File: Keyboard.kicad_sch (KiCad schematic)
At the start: 180 parts, among them SW1 SW_Push, SW10 SW_Push, SW11 SW_Push, SW12 SW_Push, SW13 SW_Push, SW14 SW_Push, SW15 SW_Push, SW16 SW_Push, SW17 SW_Push, SW18 SW_Push, SW19 SW_Push, SW2 SW_Push, SW20 SW_Push, SW21 SW_Push, SW22 SW_Push, SW23 SW_Push, SW24 SW_Push, SW25 SW_Push, SW26 SW_Push, SW27 SW_Push, SW28 SW_Push, SW29 SW_Push, SW3 SW_Push, SW30 SW_Push, SW31 SW_Push, SW32 SW_Push, SW33 SW_Push, SW34 SW_Push, SW35 SW_Push, SW36 SW_Push, SW37 SW_Push, SW38 SW_Push, SW39 SW_Push, SW4 SW_Push, SW40 SW_Push, SW41 SW_Push, SW42 SW_Push, SW43 SW_Push, SW44 SW_Push, SW45 SW_Push, SW46 SW_Push, SW47 SW_Push, SW48 SW_Push, SW49 SW_Push, SW5 SW_Push, SW50 SW_Push, SW51 SW_Push, SW52 SW_Push, SW53 SW_Push, SW54 SW_Push, SW55 SW_Push, SW56 SW_Push, SW57 SW_Push, SW58 SW_Push, SW59 SW_Push, SW6 SW_Push, SW60 SW_Push, SW61 SW_Push, SW62 SW_Push, SW63 SW_Push, SW64 SW_Push, SW65 SW_Push, SW66 SW_Push, SW67 SW_Push, SW68 SW_Push, SW69 SW_Push, SW7 SW_Push, SW70 SW_Push, SW71 SW_Push, SW72 SW_Push, SW73 SW_Push, SW74 SW_Push, SW75 SW_Push, SW76 SW_Push, SW77 SW_Push, SW78 SW_Push, SW79 SW_Push, SW8 SW_Push, SW80 SW_Push, SW81 SW_Push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

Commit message: updated footprints, didnt rlly seem to work lol
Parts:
- SW1, SW10, SW11, SW13, SW14, SW15, SW16, SW17, SW19, SW2, SW20, SW21, SW22, SW23, SW25, SW26, SW27, SW28, SW29, SW31, SW32, SW33, SW34, SW35, SW37, SW38, SW39, SW40, SW41, SW43, SW44, SW45, SW46, SW47, SW49, SW50, SW51, SW52, SW53, SW54, SW55, SW56, SW57, SW58, SW59, SW60, SW61, SW62, SW63, SW64, SW65, SW66, SW67, SW68, SW69, SW7, SW70, SW72, SW73, SW74, SW75, SW77, SW78, SW79, SW8, SW82, SW83, SW84, SW85, SW86, SW87, SW88, SW89, SW9: footprint Button_Switch_Keyboard:SW_Cherry_MX_1.00u_PCB -> Library:SW_Cherry_MX_1.00u_PCB
- SW12, SW18, SW24, SW36, SW42, SW48, SW6: footprint Button_Switch_Keyboard:SW_Cherry_MX_1.25u_PCB -> Library:SW_Cherry_MX_1.25u_PCB
- SW3, SW81: footprint Button_Switch_Keyboard:SW_Cherry_MX_1.50u_PCB -> Library:SW_Cherry_MX_1.50u_PCB
- SW30: footprint Button_Switch_Keyboard:SW_Cherry_MX_6.25u_PCB -> Library:SW_Cherry_MX_6.25u_PCB
- SW4: footprint Button_Switch_Keyboard:SW_Cherry_MX_1.75u_PCB -> Library:SW_Cherry_MX_1.75u_PCB
- SW5, SW76: footprint Button_Switch_Keyboard:SW_Cherry_MX_2.25u_PCB -> Library:SW_Cherry_MX_2.25u_PCB
- SW71: footprint Button_Switch_Keyboard:SW_Cherry_MX_2.75u_PCB -> Library:SW_Cherry_MX_2.75u_PCB
- SW80: footprint Button_Switch_Keyboard:SW_Cherry_MX_2.00u_PCB -> Library:SW_Cherry_MX_2.00u_PCB

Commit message: updating pcb
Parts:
- U1: footprint Module:RaspberryPi_Pico_Common_THT -> Library:RaspberryPi_Pico_Common_THT
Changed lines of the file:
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@@
 			)
 		)
-		(property "Footprint" "Module:RaspberryPi_Pico_Common_THT"
+		(property "Footprint" "Library:RaspberryPi_Pico_Common_THT"
 			(at 48.26 149.86 90)
 			(effects

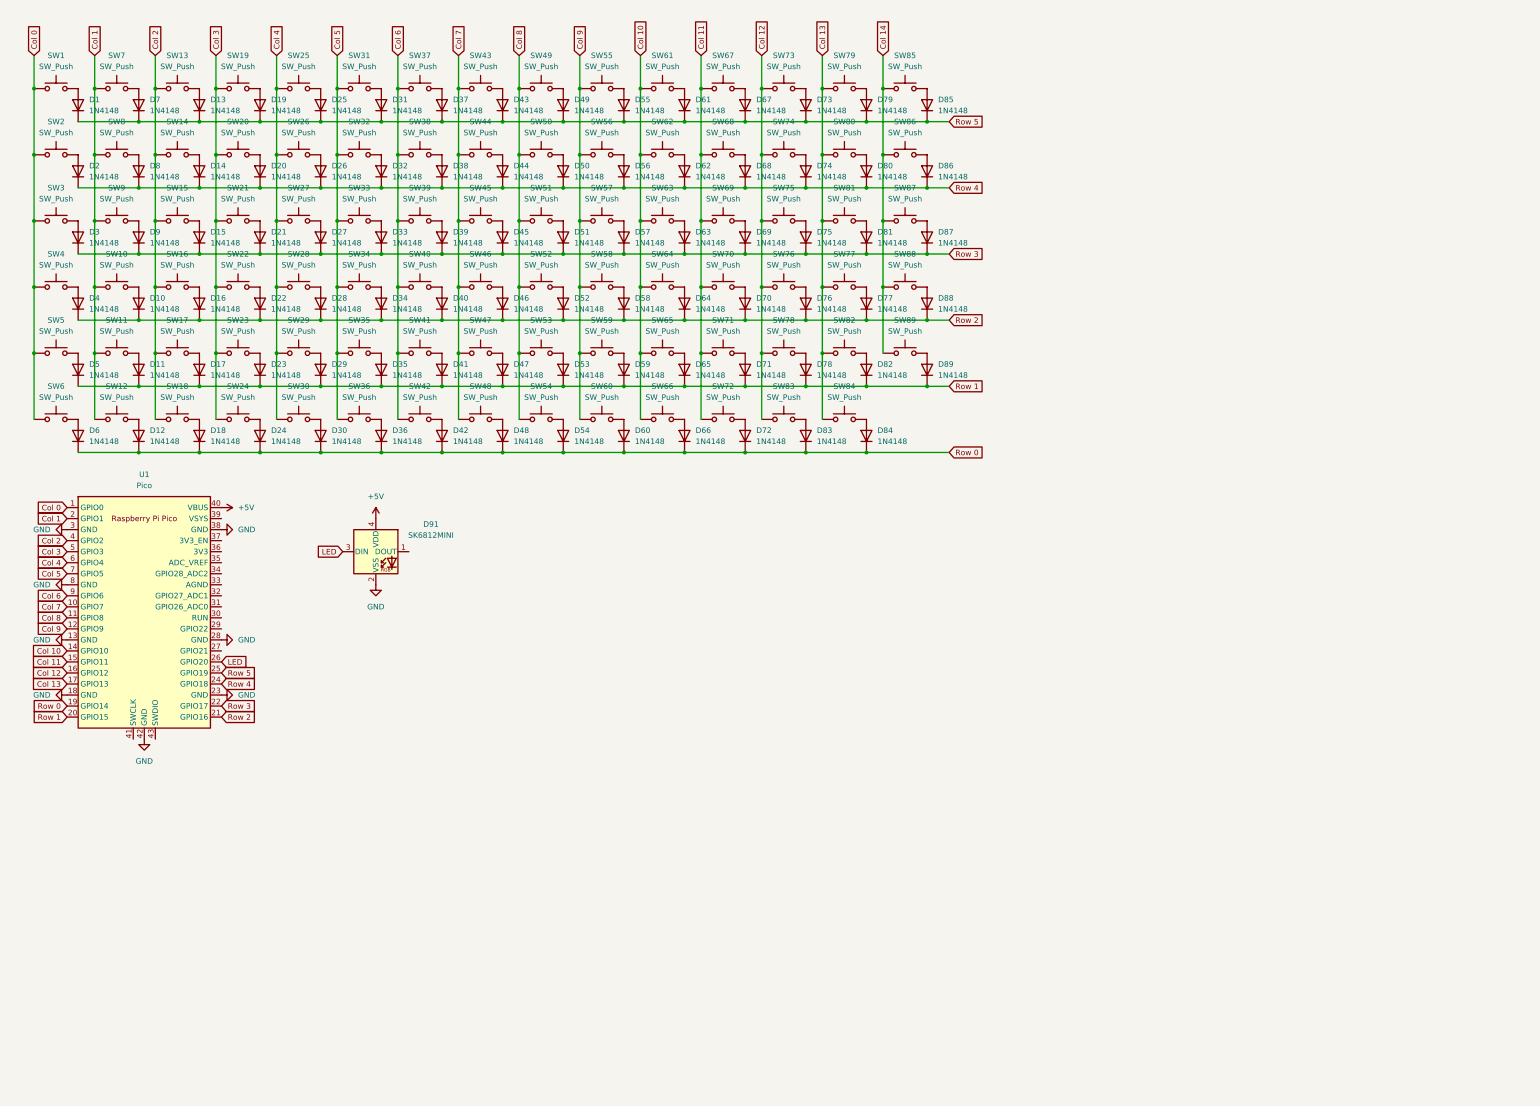
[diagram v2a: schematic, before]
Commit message: adding files
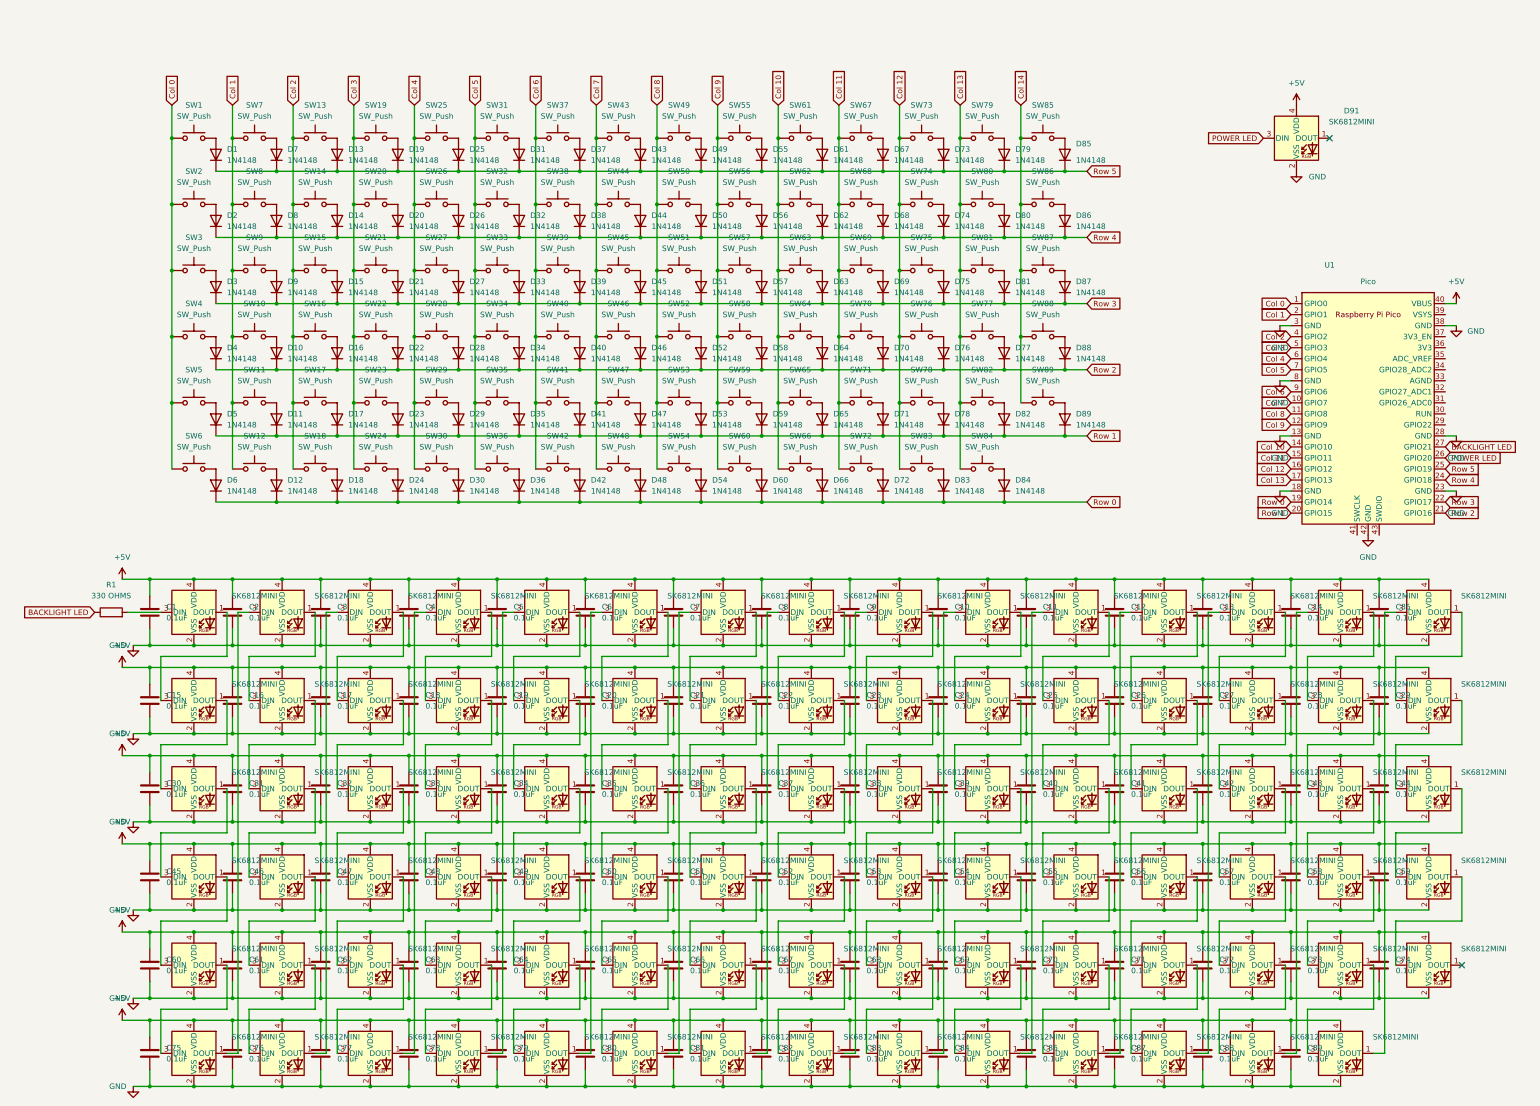
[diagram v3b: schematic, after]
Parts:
- added C1, C10, C11, C12, C13, C14, C15, C16, C17, C18, C19, C2, C20, C21, C22, C23, C24, C25, C26, C27, C28, C29, C3, C30, C31, C32, C33, C34, C35, C36, C37, C38, C39, C4, C40, C41, C42, C43, C44, C45, C46, C47, C48, C49, C5, C50, C51, C52, C53, C54, C55, C56, C57, C58, C59, C6, C60, C61, C62, C63, C64, C65, C66, C67, C68, C69, C7, C70, C71, C72, C73, C74, C75, C76, C77, C78, C79, C8, C80, C81, C82, C83, C84, C85, C86, C87, C88, C89, C9: 0.1uF, Capacitor_SMD:C_0805_2012Metric, symbol Device:C
- added D100, D101, D102, D103, D104, D105, D106, D107, D108, D109, D110, D111, D112, D113, D114, D115, D116, D117, D118, D119, D120, D121, D122, D123, D124, D125, D126, D127, D128, D129, D130, D131, D132, D133, D134, D135, D136, D137, D138, D139, D140, D141, D142, D143, D144, D145, D146, D147, D148, D149, D150, D151, D152, D153, D154, D155, D156, D157, D158, D159, D160, D161, D162, D163, D164, D165, D166, D167, D168, D169, D170, D171, D172, D173, D174, D175, D176, D177, D178, D179, D90, D92, D93, D94, D95, D96, D97, D98, D99: SK6812MINI, kai's library:MX_SK6812MINI-E_REV, symbol LED:SK6812MINI
- added R1: 330 OHMS, Resistor_SMD:R_0805_2012Metric, symbol Device:R
- D91: footprint LED_SMD:LED_SK6812MINI_PLCC4_3.5x3.5mm_P1.75mm -> kai's library:LED_SK6812MINI_PLCC4_3.5x3.5mm_P1.75mm
- U1: footprint Library:RaspberryPi_Pico_Common_THT -> kai's library:RaspberryPi_Pico_Common_THT
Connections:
- net +5V: now also C1.1, C10.1, C11.1, C12.1, C13.1, C14.1, C15.1, C16.1, C17.1, C18.1, C19.1, C2.1, C20.1, C21.1, C22.1, C23.1, C24.1, C25.1, C26.1, C27.1, C28.1, C29.1, C3.1, C30.1, C31.1, C32.1, C33.1, C34.1, C35.1, C36.1, C37.1, C38.1, C39.1, C4.1, C40.1, C41.1, C42.1, C43.1, C44.1, C45.1, C46.1, C47.1, C48.1, C49.1, C5.1, C50.1, C51.1, C52.1, C53.1, C54.1, C55.1, C56.1, C57.1, C58.1, C59.1, C6.1, C60.1, C61.1, C62.1, C63.1, C64.1, C65.1, C66.1, C67.1, C68.1, C69.1, C7.1, C70.1, C71.1, C72.1, C73.1, C74.1, C75.1, C76.1, C77.1, C78.1, C79.1, C8.1, C80.1, C81.1, C82.1, C83.1, C84.1, C85.1, C86.1, C87.1, C88.1, C89.1, C9.1, D100.4 (VDD), D101.4 (VDD), D102.4 (VDD), D103.4 (VDD), D104.4 (VDD), D105.4 (VDD), D106.4 (VDD), D107.4 (VDD), D108.4 (VDD), D109.4 (VDD), D110.4 (VDD), D111.4 (VDD), D112.4 (VDD), D113.4 (VDD), D114.4 (VDD), D115.4 (VDD), D116.4 (VDD), D117.4 (VDD), D118.4 (VDD), D119.4 (VDD), D120.4 (VDD), D121.4 (VDD), D122.4 (VDD), D123.4 (VDD), D124.4 (VDD), D125.4 (VDD), D126.4 (VDD), D127.4 (VDD), D128.4 (VDD), D129.4 (VDD), D130.4 (VDD), D131.4 (VDD), D132.4 (VDD), D133.4 (VDD), D134.4 (VDD), D135.4 (VDD), D136.4 (VDD), D137.4 (VDD), D138.4 (VDD), D139.4 (VDD), D140.4 (VDD), D141.4 (VDD), D142.4 (VDD), D143.4 (VDD), D144.4 (VDD), D145.4 (VDD), D146.4 (VDD), D147.4 (VDD), D148.4 (VDD), D149.4 (VDD), D150.4 (VDD), D151.4 (VDD), D152.4 (VDD), D153.4 (VDD), D154.4 (VDD), D155.4 (VDD), D156.4 (VDD), D157.4 (VDD), D158.4 (VDD), D159.4 (VDD), D160.4 (VDD), D161.4 (VDD), D162.4 (VDD), D163.4 (VDD), D164.4 (VDD), D165.4 (VDD), D166.4 (VDD), D167.4 (VDD), D168.4 (VDD), D169.4 (VDD), D170.4 (VDD), D171.4 (VDD), D172.4 (VDD), D173.4 (VDD), D174.4 (VDD), D175.4 (VDD), D176.4 (VDD), D177.4 (VDD), D178.4 (VDD), D179.4 (VDD), D90.4 (VDD), D92.4 (VDD), D93.4 (VDD), D94.4 (VDD), D95.4 (VDD), D96.4 (VDD), D97.4 (VDD), D98.4 (VDD), D99.4 (VDD)
- net GND: now also C1.2, C10.2, C11.2, C12.2, C13.2, C14.2, C15.2, C16.2, C17.2, C18.2, C19.2, C2.2, C20.2, C21.2, C22.2, C23.2, C24.2, C25.2, C26.2, C27.2, C28.2, C29.2, C3.2, C30.2, C31.2, C32.2, C33.2, C34.2, C35.2, C36.2, C37.2, C38.2, C39.2, C4.2, C40.2, C41.2, C42.2, C43.2, C44.2, C45.2, C46.2, C47.2, C48.2, C49.2, C5.2, C50.2, C51.2, C52.2, C53.2, C54.2, C55.2, C56.2, C57.2, C58.2, C59.2, C6.2, C60.2, C61.2, C62.2, C63.2, C64.2, C65.2, C66.2, C67.2, C68.2, C69.2, C7.2, C70.2, C71.2, C72.2, C73.2, C74.2, C75.2, C76.2, C77.2, C78.2, C79.2, C8.2, C80.2, C81.2, C82.2, C83.2, C84.2, C85.2, C86.2, C87.2, C88.2, C89.2, C9.2, D100.2 (VSS), D101.2 (VSS), D102.2 (VSS), D103.2 (VSS), D104.2 (VSS), D105.2 (VSS), D106.2 (VSS), D107.2 (VSS), D108.2 (VSS), D109.2 (VSS), D110.2 (VSS), D111.2 (VSS), D112.2 (VSS), D113.2 (VSS), D114.2 (VSS), D115.2 (VSS), D116.2 (VSS), D117.2 (VSS), D118.2 (VSS), D119.2 (VSS), D120.2 (VSS), D121.2 (VSS), D122.2 (VSS), D123.2 (VSS), D124.2 (VSS), D125.2 (VSS), D126.2 (VSS), D127.2 (VSS), D128.2 (VSS), D129.2 (VSS), D130.2 (VSS), D131.2 (VSS), D132.2 (VSS), D133.2 (VSS), D134.2 (VSS), D135.2 (VSS), D136.2 (VSS), D137.2 (VSS), D138.2 (VSS), D139.2 (VSS), D140.2 (VSS), D141.2 (VSS), D142.2 (VSS), D143.2 (VSS), D144.2 (VSS), D145.2 (VSS), D146.2 (VSS), D147.2 (VSS), D148.2 (VSS), D149.2 (VSS), D150.2 (VSS), D151.2 (VSS), D152.2 (VSS), D153.2 (VSS), D154.2 (VSS), D155.2 (VSS), D156.2 (VSS), D157.2 (VSS), D158.2 (VSS), D159.2 (VSS), D160.2 (VSS), D161.2 (VSS), D162.2 (VSS), D163.2 (VSS), D164.2 (VSS), D165.2 (VSS), D166.2 (VSS), D167.2 (VSS), D168.2 (VSS), D169.2 (VSS), D170.2 (VSS), D171.2 (VSS), D172.2 (VSS), D173.2 (VSS), D174.2 (VSS), D175.2 (VSS), D176.2 (VSS), D177.2 (VSS), D178.2 (VSS), D179.2 (VSS), D90.2 (VSS), D92.2 (VSS), D93.2 (VSS), D94.2 (VSS), D95.2 (VSS), D96.2 (VSS), D97.2 (VSS), D98.2 (VSS), D99.2 (VSS)
- net BACKLIGHT LED: now reaches U1.27 (GPIO21)
- net BACKLIGHT LED: now also R1.1
- net LED renamed POWER LED
- new net: D127.1 (DOUT), D128.3 (DIN)
- new net: D126.1 (DOUT), D127.3 (DIN)
- new net: D103.1 (DOUT), D104.3 (DIN)
- new net: D102.1 (DOUT), D103.3 (DIN)
- new net: D90.3 (DIN), D92.1 (DOUT)
- new net: D92.3 (DIN), R1.2
- new net: D132.1 (DOUT), D133.3 (DIN)
- new net: D131.1 (DOUT), D132.3 (DIN)
- new net: D112.1 (DOUT), D113.3 (DIN)
- new net: D111.1 (DOUT), D112.3 (DIN)
- new net: D125.1 (DOUT), D126.3 (DIN)
- new net: D148.1 (DOUT), D149.3 (DIN)
- new net: D147.1 (DOUT), D148.3 (DIN)
- new net: D145.1 (DOUT), D146.3 (DIN)
- new net: D144.1 (DOUT), D145.3 (DIN)
- new net: D118.1 (DOUT), D119.3 (DIN)
- new net: D117.1 (DOUT), D118.3 (DIN)
- new net: D133.1 (DOUT), D134.3 (DIN)
- new net: D128.1 (DOUT), D129.3 (DIN)
- new net: D169.1 (DOUT), D170.3 (DIN)
- new net: D168.1 (DOUT), D169.3 (DIN)
- new net: D178.1 (DOUT), D179.3 (DIN)
- new net: D108.1 (DOUT), D109.3 (DIN)
- new net: D107.1 (DOUT), D108.3 (DIN)
- new net: D176.1 (DOUT), D177.3 (DIN)
- new net: D175.1 (DOUT), D176.3 (DIN)
- new net: D121.1 (DOUT), D122.3 (DIN)
- new net: D120.1 (DOUT), D121.3 (DIN)
- new net: D113.1 (DOUT), D114.3 (DIN)
- new net: D174.1 (DOUT), D175.3 (DIN)
- new net: D173.1 (DOUT), D174.3 (DIN)
- new net: D159.1 (DOUT), D160.3 (DIN)
- new net: D158.1 (DOUT), D159.3 (DIN)
- new net: D119.1 (DOUT), D120.3 (DIN)
- new net: D109.1 (DOUT), D110.3 (DIN)
- new net: D137.1 (DOUT), D138.3 (DIN)
- new net: D136.1 (DOUT), D137.3 (DIN)
- new net: D151.1 (DOUT), D152.3 (DIN)
- new net: D150.1 (DOUT), D151.3 (DIN)
- new net: D161.1 (DOUT), D162.3 (DIN)
- new net: D160.1 (DOUT), D161.3 (DIN)
- new net: D123.1 (DOUT), D124.3 (DIN)
- new net: D122.1 (DOUT), D123.3 (DIN)
- new net: D135.1 (DOUT), D136.3 (DIN)
- new net: D134.1 (DOUT), D135.3 (DIN)
- new net: D124.1 (DOUT), D125.3 (DIN)
- new net: D164.1 (DOUT), D165.3 (DIN)
- new net: D163.1 (DOUT), D164.3 (DIN)
- new net: D105.1 (DOUT), D106.3 (DIN)
- new net: D104.1 (DOUT), D105.3 (DIN)
- new net: D177.1 (DOUT), D178.3 (DIN)
- new net: D100.1 (DOUT), D101.3 (DIN)
- new net: D100.3 (DIN), D99.1 (DOUT)
- new net: D171.1 (DOUT), D172.3 (DIN)
- new net: D170.1 (DOUT), D171.3 (DIN)
- new net: D157.1 (DOUT), D158.3 (DIN)
- new net: D165.1 (DOUT), D166.3 (DIN)
- new net: D114.1 (DOUT), D115.3 (DIN)
- new net: D106.1 (DOUT), D107.3 (DIN)
- new net: D153.1 (DOUT), D154.3 (DIN)
- new net: D152.1 (DOUT), D153.3 (DIN)
- new net: D172.1 (DOUT), D173.3 (DIN)
- new net: D110.1 (DOUT), D111.3 (DIN)
- new net: D139.1 (DOUT), D140.3 (DIN)
- new net: D138.1 (DOUT), D139.3 (DIN)
- new net: D98.1 (DOUT), D99.3 (DIN)
- new net: D143.1 (DOUT), D144.3 (DIN)
- new net: D142.1 (DOUT), D143.3 (DIN)
- new net: D115.1 (DOUT), D116.3 (DIN)
- new net: D90.1 (DOUT), D93.3 (DIN)
- new net: D116.1 (DOUT), D117.3 (DIN)
- new net: D167.1 (DOUT), D168.3 (DIN)
- new net: D166.1 (DOUT), D167.3 (DIN)
- new net: D95.1 (DOUT), D96.3 (DIN)
- new net: D94.1 (DOUT), D95.3 (DIN)
- new net: D149.1 (DOUT), D150.3 (DIN)
- new net: D93.1 (DOUT), D94.3 (DIN)
- new net: D101.1 (DOUT), D102.3 (DIN)
- new net: D97.1 (DOUT), D98.3 (DIN)
- new net: D96.1 (DOUT), D97.3 (DIN)
- new net: D130.1 (DOUT), D131.3 (DIN)
- new net: D146.1 (DOUT), D147.3 (DIN)
- new net: D154.1 (DOUT), D155.3 (DIN)
- new net: D162.1 (DOUT), D163.3 (DIN)
- new net: D129.1 (DOUT), D130.3 (DIN)
- new net: D156.1 (DOUT), D157.3 (DIN)
- new net: D141.1 (DOUT), D142.3 (DIN)
- new net: D155.1 (DOUT), D156.3 (DIN)
- new net: D140.1 (DOUT), D141.3 (DIN)
- no-connect marks 0 -> 2
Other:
- moved on the sheet: D1, D10, D11, D12, D13, D14, D15, D16, D17, D18, D19, D2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

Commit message: added 3d models to keys
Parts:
- SW1, SW10, SW11, SW13, SW14, SW15, SW16, SW17, SW19, SW2, SW20, SW21, SW22, SW23, SW25, SW26, SW27, SW28, SW29, SW31, SW32, SW33, SW34, SW35, SW37, SW38, SW39, SW40, SW41, SW43, SW44, SW45, SW46, SW47, SW49, SW50, SW51, SW52, SW53, SW54, SW55, SW56, SW57, SW58, SW59, SW60, SW61, SW62, SW63, SW64, SW65, SW66, SW67, SW68, SW69, SW7, SW70, SW72, SW73, SW74, SW75, SW77, SW78, SW79, SW8, SW82, SW83, SW84, SW85, SW86, SW87, SW88, SW89, SW9: footprint Library:SW_Cherry_MX_1.00u_PCB -> kai's library:SW_Cherry_MX_1.00u_PCB
- SW80: footprint Library:SW_Cherry_MX_2.00u_PCB -> Button_Switch_Keyboard:SW_Cherry_MX_2.00u_PCB
- SW81: footprint Library:SW_Cherry_MX_1.50u_PCB -> kai's library:SW_Cherry_MX_1.00u_PCB

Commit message: adding some 3d models
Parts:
- SW3: footprint Library:SW_Cherry_MX_1.50u_PCB -> kai's library:SW_Cherry_MX_1.50u_PCB
- SW4: footprint Library:SW_Cherry_MX_1.75u_PCB -> kai's library:SW_Cherry_MX_1.75u_PCB
- SW5, SW76: footprint Library:SW_Cherry_MX_2.25u_PCB -> kai's library:SW_Cherry_MX_2.25u_PCB
- SW71: footprint Library:SW_Cherry_MX_2.75u_PCB -> kai's library:SW_Cherry_MX_2.25u_PCB
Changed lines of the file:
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@@
 			)
 		)
-		(property "Footprint" "Library:SW_Cherry_MX_2.75u_PCB"
+		(property "Footprint" "kai's library:SW_Cherry_MX_2.25u_PCB"
 			(at 213.36 96.52 0)
 			(effects
@@
 			)
 		)
-		(property "Footprint" "Library:SW_Cherry_MX_2.25u_PCB"
+		(property "Footprint" "kai's library:SW_Cherry_MX_2.25u_PCB"
 			(at 227.33 81.28 0)
 			(effects
@@
 			)
 		)
-		(property "Footprint" "Library:SW_Cherry_MX_2.25u_PCB"
+		(property "Footprint" "kai's library:SW_Cherry_MX_2.25u_PCB"
 			(at 59.69 96.52 0)
 			(effects
@@
 			)
 		)
-		(property "Footprint" "Library:SW_Cherry_MX_1.50u_PCB"
+		(property "Footprint" "kai's library:SW_Cherry_MX_1.50u_PCB"
 			(at 59.69 66.04 0)
 			(effects
@@
 			)
 		)
-		(property "Footprint" "Library:SW_Cherry_MX_1.75u_PCB"
+		(property "Footprint" "kai's library:SW_Cherry_MX_1.75u_PCB"
 			(at 59.69 81.28 0)
 			(effects

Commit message: 3d models and updated footprints
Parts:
- SW12, SW18, SW24, SW36, SW42, SW48, SW6: footprint Library:SW_Cherry_MX_1.25u_PCB -> kai's library:SW_Cherry_MX_1.25u_PCB
- SW30: footprint Library:SW_Cherry_MX_6.25u_PCB -> kai's library:SW_Cherry_MX_6.25u_PCB
- SW71: footprint kai's library:SW_Cherry_MX_2.25u_PCB -> kai's library:SW_Cherry_MX_2.75u_PCB
- SW80: footprint Button_Switch_Keyboard:SW_Cherry_MX_2.00u_PCB -> kai's library:SW_Cherry_MX_2.00u_PCB
- SW81: footprint kai's library:SW_Cherry_MX_1.00u_PCB -> kai's library:SW_Cherry_MX_1.50u_PCB
- U1: footprint kai's library:RaspberryPi_Pico_Common_THT -> kai's library:RaspberryPi_Pico_Common_THT_BACKSIDE
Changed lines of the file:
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@@
 			)
 		)
-		(property "Footprint" "kai's library:SW_Cherry_MX_1.00u_PCB"
+		(property "Footprint" "kai's library:SW_Cherry_MX_1.50u_PCB"
 			(at 241.3 66.04 0)
 			(effects
@@
 			)
 		)
-		(property "Footprint" "Library:SW_Cherry_MX_1.25u_PCB"
+		(property "Footprint" "kai's library:SW_Cherry_MX_1.25u_PCB"
 			(at 157.48 111.76 0)
 			(effects
@@
 			)
 		)
-		(property "Footprint" "kai's library:SW_Cherry_MX_2.25u_PCB"
+		(property "Footprint" "kai's library:SW_Cherry_MX_2.75u_PCB"
 			(at 213.36 96.52 0)
 			(effects
@@
 			)
 		)
-		(property "Footprint" "Library:SW_Cherry_MX_6.25u_PCB"
+		(property "Footprint" "kai's library:SW_Cherry_MX_6.25u_PCB"
 			(at 115.57 111.76 0)
 			(effects
@@
 			)
 		)
-		(property "Footprint" "Library:SW_Cherry_MX_1.25u_PCB"
+		(property "Footprint" "kai's library:SW_Cherry_MX_1.25u_PCB"
 			(at 129.54 111.76 0)
 			(effects
@@
 			)
 		)
-		(property "Footprint" "kai's library:RaspberryPi_Pico_Common_THT"
+		(property "Footprint" "kai's library:RaspberryPi_Pico_Common_THT_BACKSIDE"
 			(at 330.2 102.87 90)
 			(effects
@@
 			)
 		)
-		(property "Footprint" "Library:SW_Cherry_MX_1.25u_PCB"
+		(property "Footprint" "kai's library:SW_Cherry_MX_1.25u_PCB"
 			(at 101.6 111.76 0)
 			(effects
@@
 			)
 		)
-		(property "Footprint" "Library:SW_Cherry_MX_1.25u_PCB"
+		(property "Footprint" "kai's library:SW_Cherry_MX_1.25u_PCB"
 			(at 143.51 111.76 0)
 			(effects
@@
 			)
 		)
-		(property "Footprint" "Library:SW_Cherry_MX_1.25u_PCB"
+		(property "Footprint" "kai's library:SW_Cherry_MX_1.25u_PCB"
 			(at 59.69 111.76 0)
 			(effects
@@
 			)
 		)
-		(property "Footprint" "Button_Switch_Keyboard:SW_Cherry_MX_2.00u_PCB"
+		(property "Footprint" "kai's library:SW_Cherry_MX_2.00u_PCB"
 			(at 241.3 50.8 0)
 			(effects
@@
 			)
 		)
-		(property "Footprint" "Library:SW_Cherry_MX_1.25u_PCB"
+		(property "Footprint" "kai's library:SW_Cherry_MX_1.25u_PCB"
 			(at 73.66 111.76 0)
 			(effects
@@
 			)
 		)
-		(property "Footprint" "Library:SW_Cherry_MX_1.25u_PCB"
+		(property "Footprint" "kai's library:SW_Cherry_MX_1.25u_PCB"
 			(at 87.63 111.76 0)
 			(effects
